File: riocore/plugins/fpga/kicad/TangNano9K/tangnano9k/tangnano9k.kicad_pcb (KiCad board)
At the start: 2 copper layers, 28 x 72.2 mm, 1 part, among them U1 Tang_Nano_9k

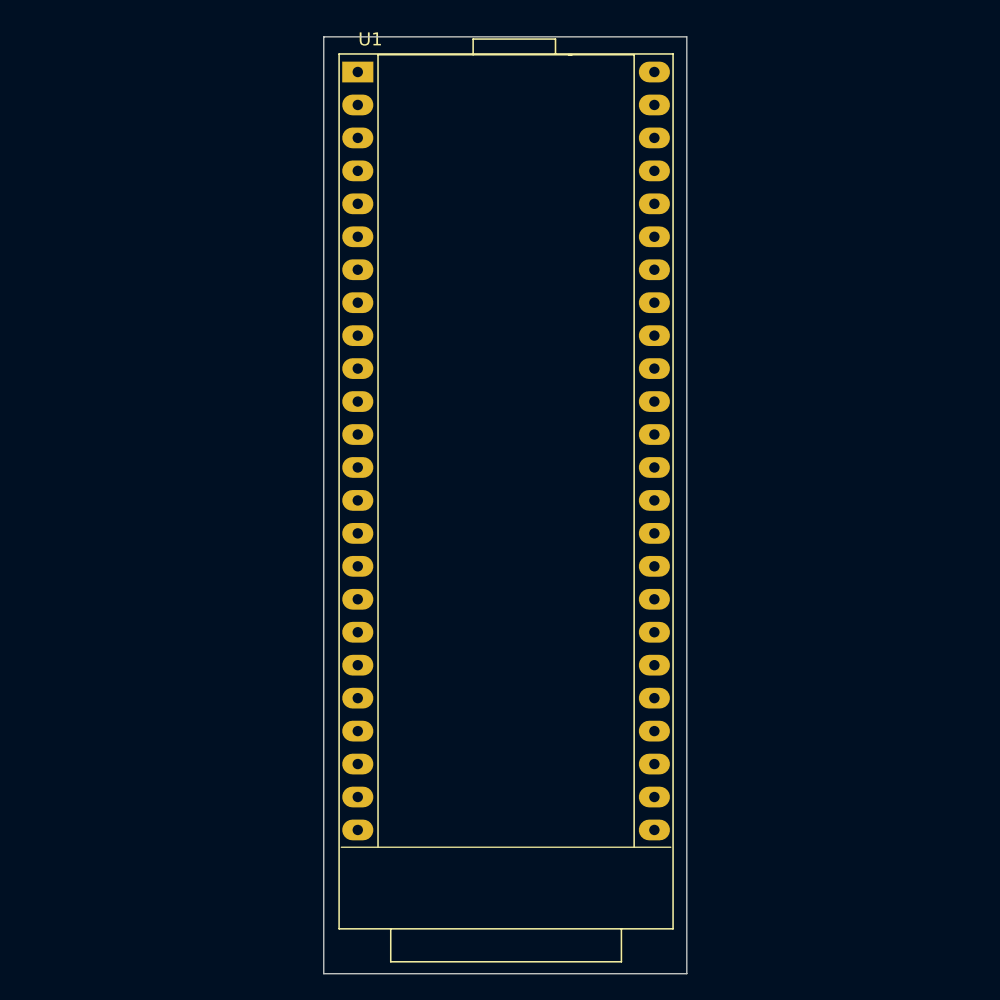
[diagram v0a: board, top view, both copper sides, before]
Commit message: kicad: pos/rotate/image
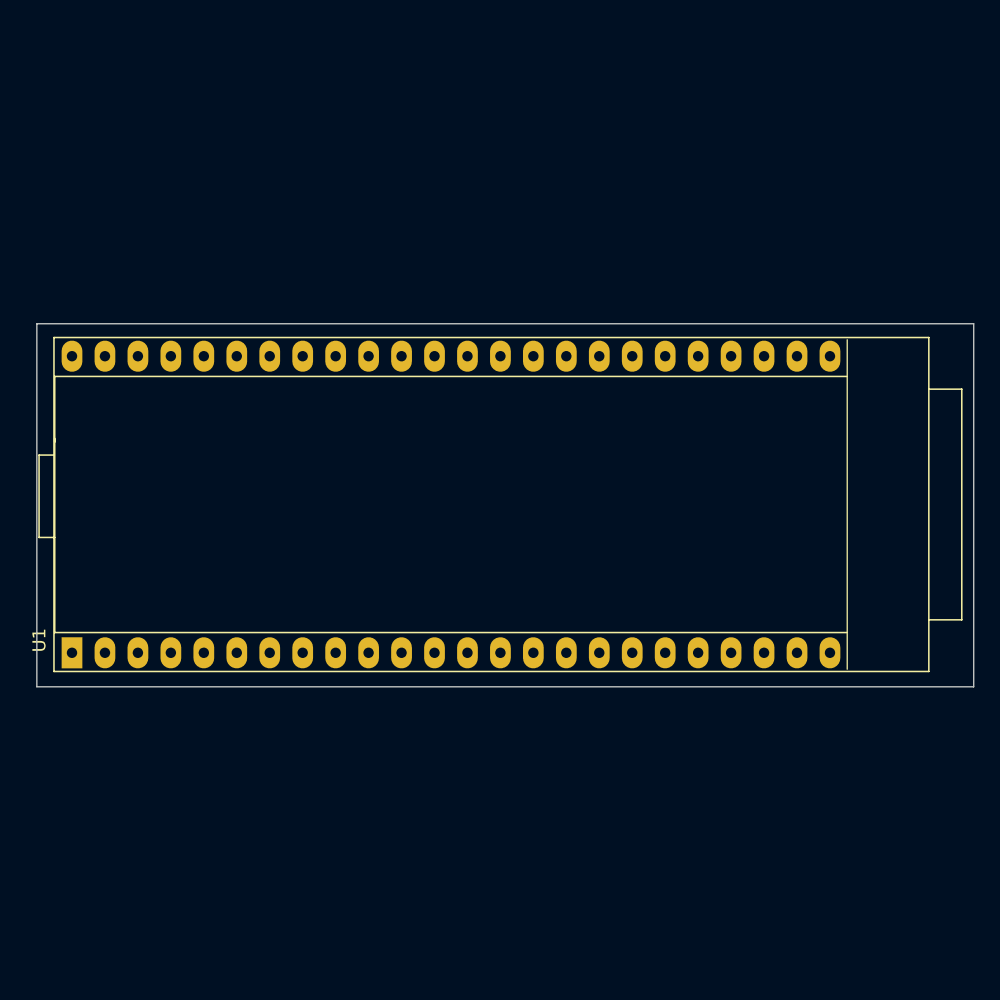
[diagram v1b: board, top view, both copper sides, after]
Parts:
- moved U1 49.9 mm to (104.0, 96.0), turned to 90 degrees
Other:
- board size 28 x 72.2 mm -> 72.2 x 28 mm

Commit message: kicad: use image selection
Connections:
- U1 pad 1: unconnected-(U1-38_IOB31B_TF_CS-Pad1) -> 38
- U1 pad 10: unconnected-(U1-30_IOB13B-Pad10) -> 30
- U1 pad 11: unconnected-(U1-33_IOB23A_RGB_DE-Pad11) -> 33
- U1 pad 12: unconnected-(U1-34_IOB23B_RGB_VS-Pad12) -> 34
- U1 pad 13: unconnected-(U1-40_IOB33B_RGB_HS-Pad13) -> 40
- U1 pad 14: unconnected-(U1-35_IOB29A_RGB_CK_GCLKT_4-Pad14) -> 35
- U1 pad 15: unconnected-(U1-41_IOB41A_RGB_B7-Pad15) -> 41
- U1 pad 16: unconnected-(U1-42_IOB41B_RGB_B6-Pad16) -> 42
- U1 pad 17: unconnected-(U1-51_IOR17B_RGB_B5_GCLKC_3-Pad17) -> 51
- U1 pad 18: unconnected-(U1-53_IOB15B_RGB_B4-Pad18) -> 53
- U1 pad 19: unconnected-(U1-54_IOB15A_RGB_B3-Pad19) -> 54
- U1 pad 2: unconnected-(U1-37_IOB31A_TF_MOSI-Pad2) -> 37
- U1 pad 20: unconnected-(U1-55_IOR14B_RGB_G7-Pad20) -> 55
- U1 pad 21: unconnected-(U1-56_IOR14A_RGB_G6-Pad21) -> 56
- U1 pad 22: unconnected-(U1-57_IOR13A_RGB_G5-Pad22) -> 57
- U1 pad 23: unconnected-(U1-68_IOT42B_RGB_G4_HDMI_CKN-Pad23) -> 68
- U1 pad 24: unconnected-(U1-69_IOT42A_RGB_G3_HDMI_CKP-Pad24) -> 69
- U1 pad 27: unconnected-(U1-RGB_INIT_IOB15B_32-Pad27) -> 32
- U1 pad 28: unconnected-(U1-RGB_INIT_IOB15A_31-Pad28) -> 31
- U1 pad 29: unconnected-(U1-SPILCD_RS_IOR24A_49-Pad29) -> 49
- U1 pad 3: unconnected-(U1-36_IOB29B_TF_SCLK_GCLKC_4-Pad3) -> 36
- U1 pad 30: unconnected-(U1-SPILCD_CS_IOR24B_48-Pad30) -> 48
- U1 pad 32: unconnected-(U1-HDMI_D0N_RGB_G2_IOT41B_70-Pad32) -> 70
- U1 pad 33: unconnected-(U1-HDMI_D0P_RGB_R7_IOT41A_71-Pad33) -> 71
- U1 pad 34: unconnected-(U1-HDMI_D1N_RGB_R6_IOT39B_72-Pad34) -> 72
- U1 pad 35: unconnected-(U1-HDMI_D1P_RGB_R5_IOT39A_73-Pad35) -> 73
- U1 pad 36: unconnected-(U1-HDMI_D2N_RGB_R4_IOT38B_74-Pad36) -> 74
- U1 pad 37: unconnected-(U1-HDMI_D2P_RGB_R3_IOT38A_75-Pad37) -> 75
- U1 pad 38: unconnected-(U1-SPILCD_CK_IOT37B_76-Pad38) -> 76
- U1 pad 39: unconnected-(U1-SPILCD_MO_IOT37A_77-Pad39) -> 77
- U1 pad 4: unconnected-(U1-39_IOB33A_TF_MISO-Pad4) -> 39
- U1 pad 40: unconnected-(U1-IOT12B_79-Pad40) -> 79
- U1 pad 41: unconnected-(U1-IOT12A_80-Pad41) -> 80
- U1 pad 42: unconnected-(U1-IOT11B_81-Pad42) -> 81
- U1 pad 43: unconnected-(U1-IOT11A_82-Pad43) -> 82
- U1 pad 44: unconnected-(U1-IOT10B_83-Pad44) -> 83
- U1 pad 45: unconnected-(U1-IOT10A_84-Pad45) -> 84
- U1 pad 46: unconnected-(U1-IOT8B_85-Pad46) -> 85
- U1 pad 47: unconnected-(U1-RGB_BL_IOT8A_86-Pad47) -> 86
- U1 pad 48: unconnected-(U1-RGB_INIT_IOR5A_63-Pad48) -> 63
- U1 pad 5: unconnected-(U1-25_IOB8A-Pad5) -> 25
- U1 pad 6: unconnected-(U1-26_IOB8B-Pad6) -> 26
- U1 pad 7: unconnected-(U1-27_IOB11A-Pad7) -> 27
- U1 pad 8: unconnected-(U1-28_IOB11B-Pad8) -> 28
- U1 pad 9: unconnected-(U1-29_IOB13A-Pad9) -> 29

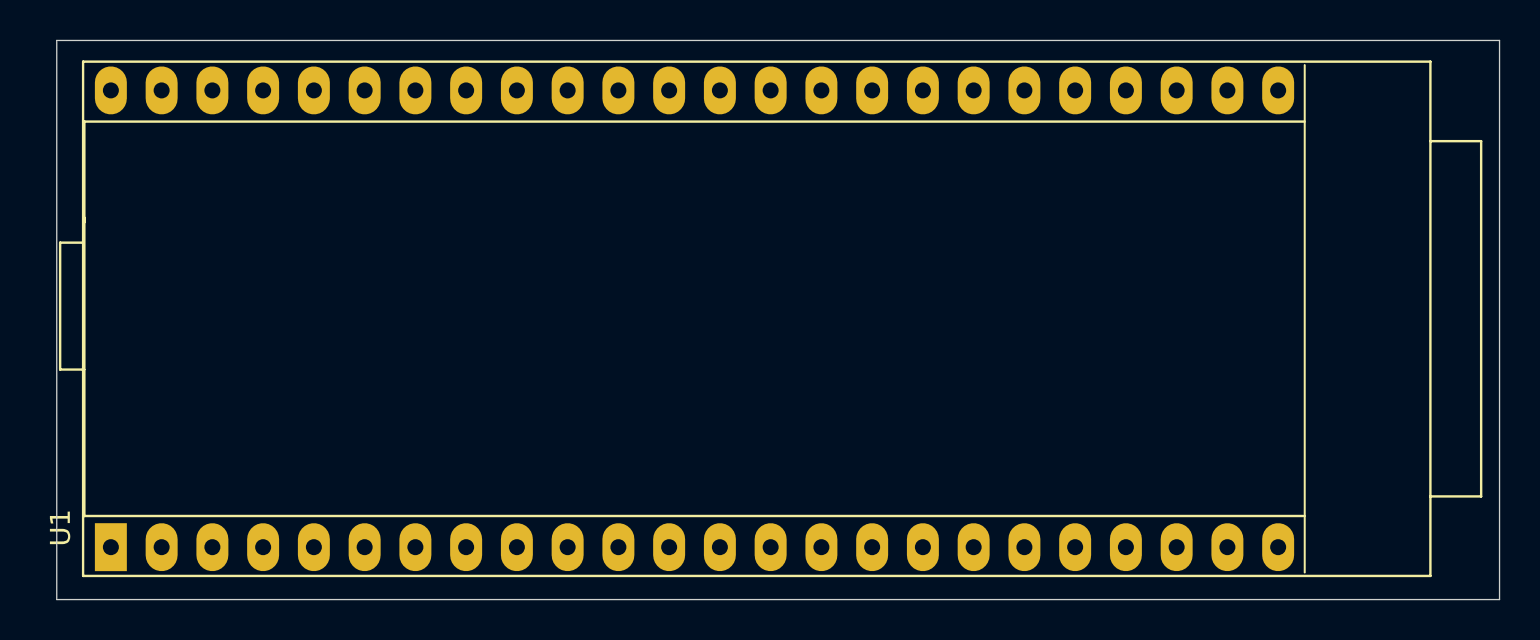
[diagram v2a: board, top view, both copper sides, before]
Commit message: kicad: pin pos
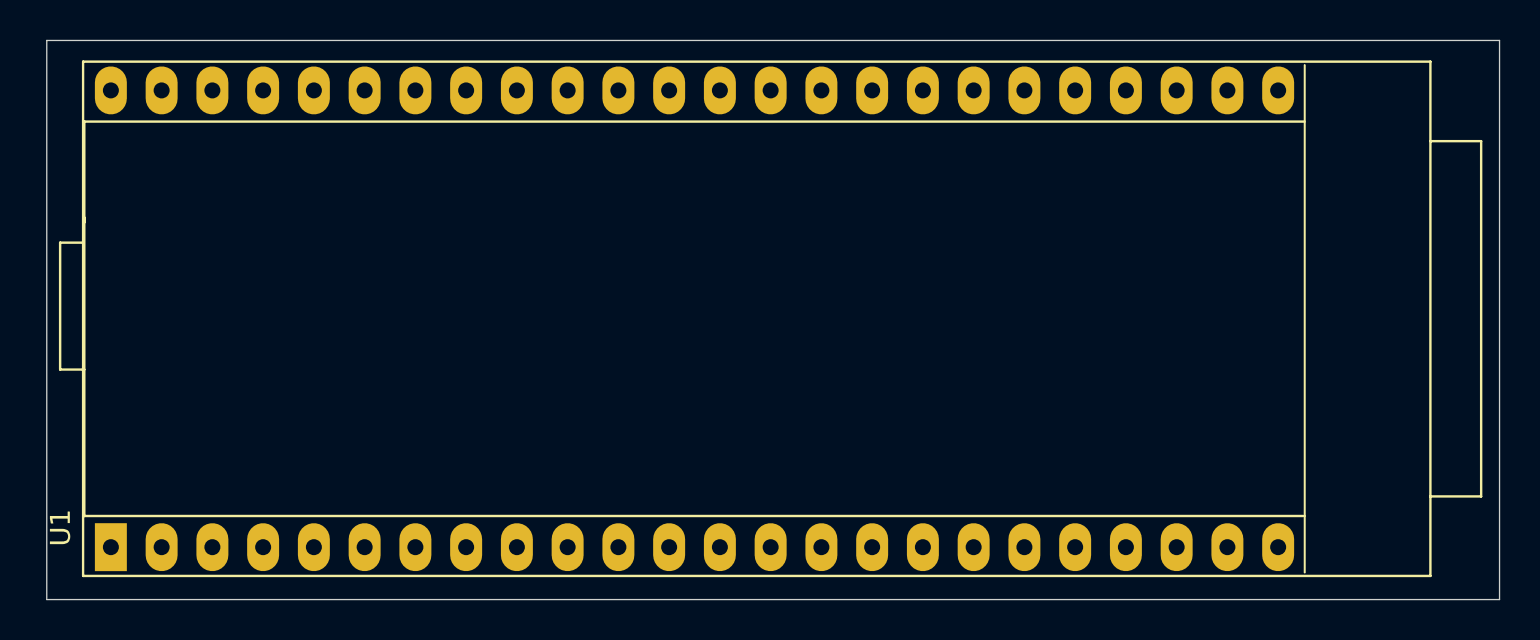
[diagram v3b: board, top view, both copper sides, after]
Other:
- board size 72.2 x 28 mm -> 72.7 x 28 mm
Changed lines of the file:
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@@
 	)
 	(gr_rect
-		(start 101.2645 70.6445)
+		(start 100.7645 70.6445)
 		(end 173.4735 98.6265)
 		(stroke
